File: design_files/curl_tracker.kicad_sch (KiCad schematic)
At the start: 38 parts, among them J1 JST-PH, J2 USB_C_Receptacle, J3 SSD1306 OLED, J4 JST-PH, Q1 DMP2035, Q2 AO3400A, SW1 SW_Push, SW2 SW_Push, SW3 SW_Push, U1 AP2112K-3.3, U2 ESP32-C3-MINI-1, U3 MCP73831-2-OT, U4 BMI270, U5 USBLC6-2SC6

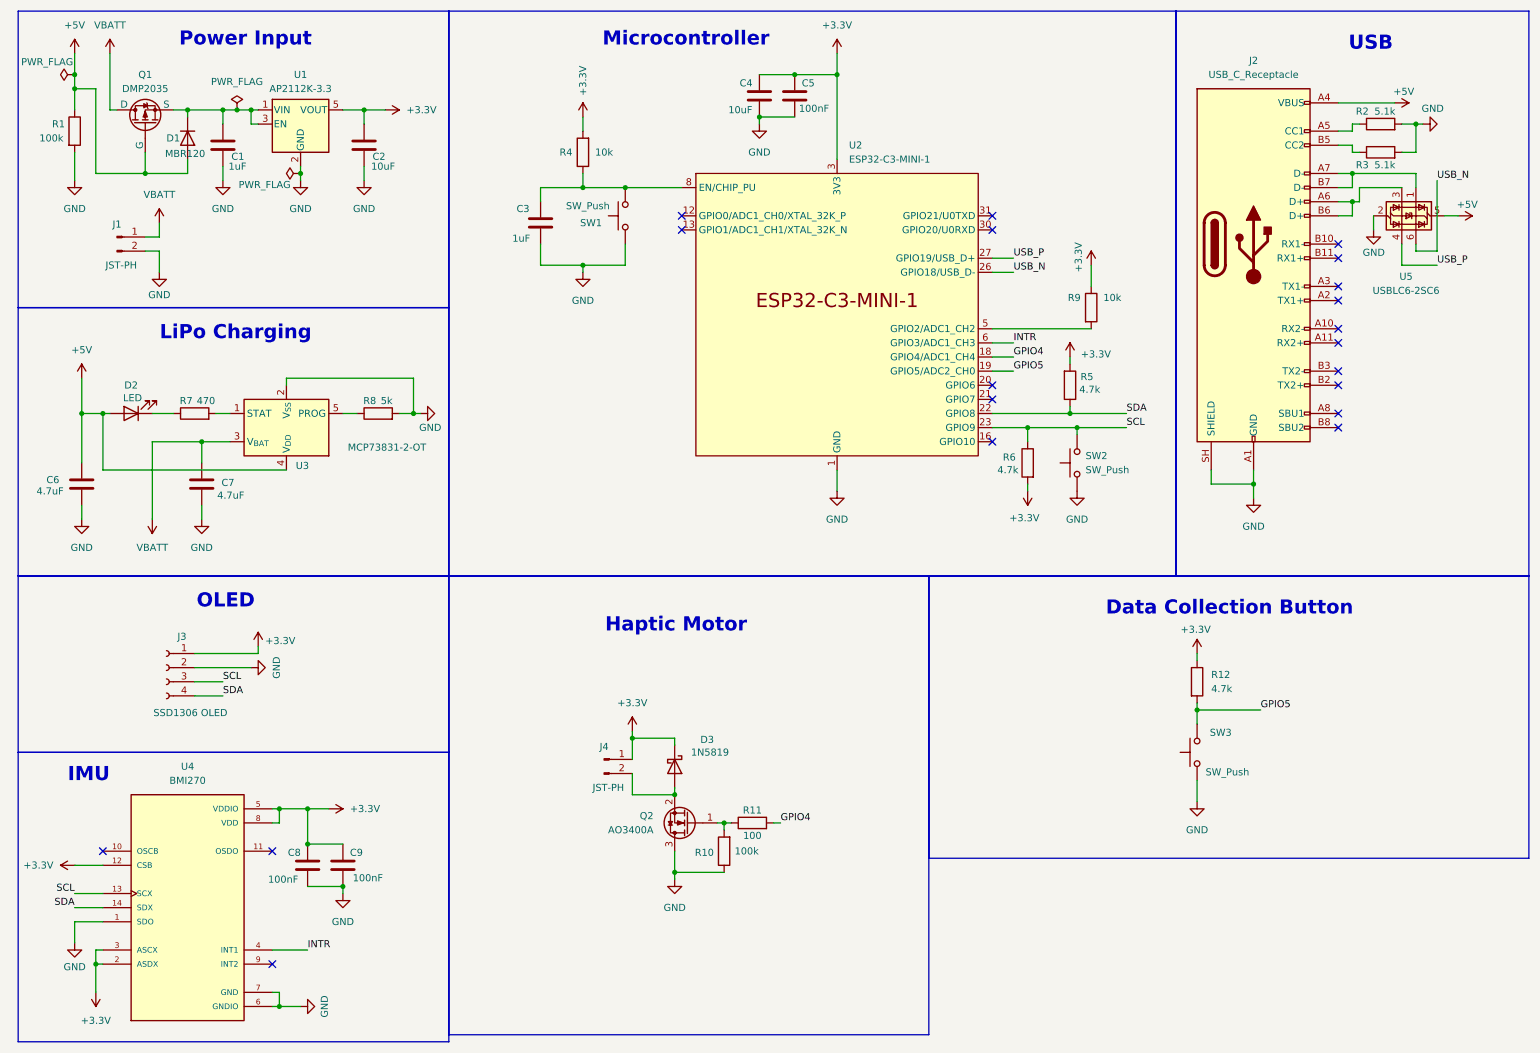
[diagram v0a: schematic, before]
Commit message: finished schematic
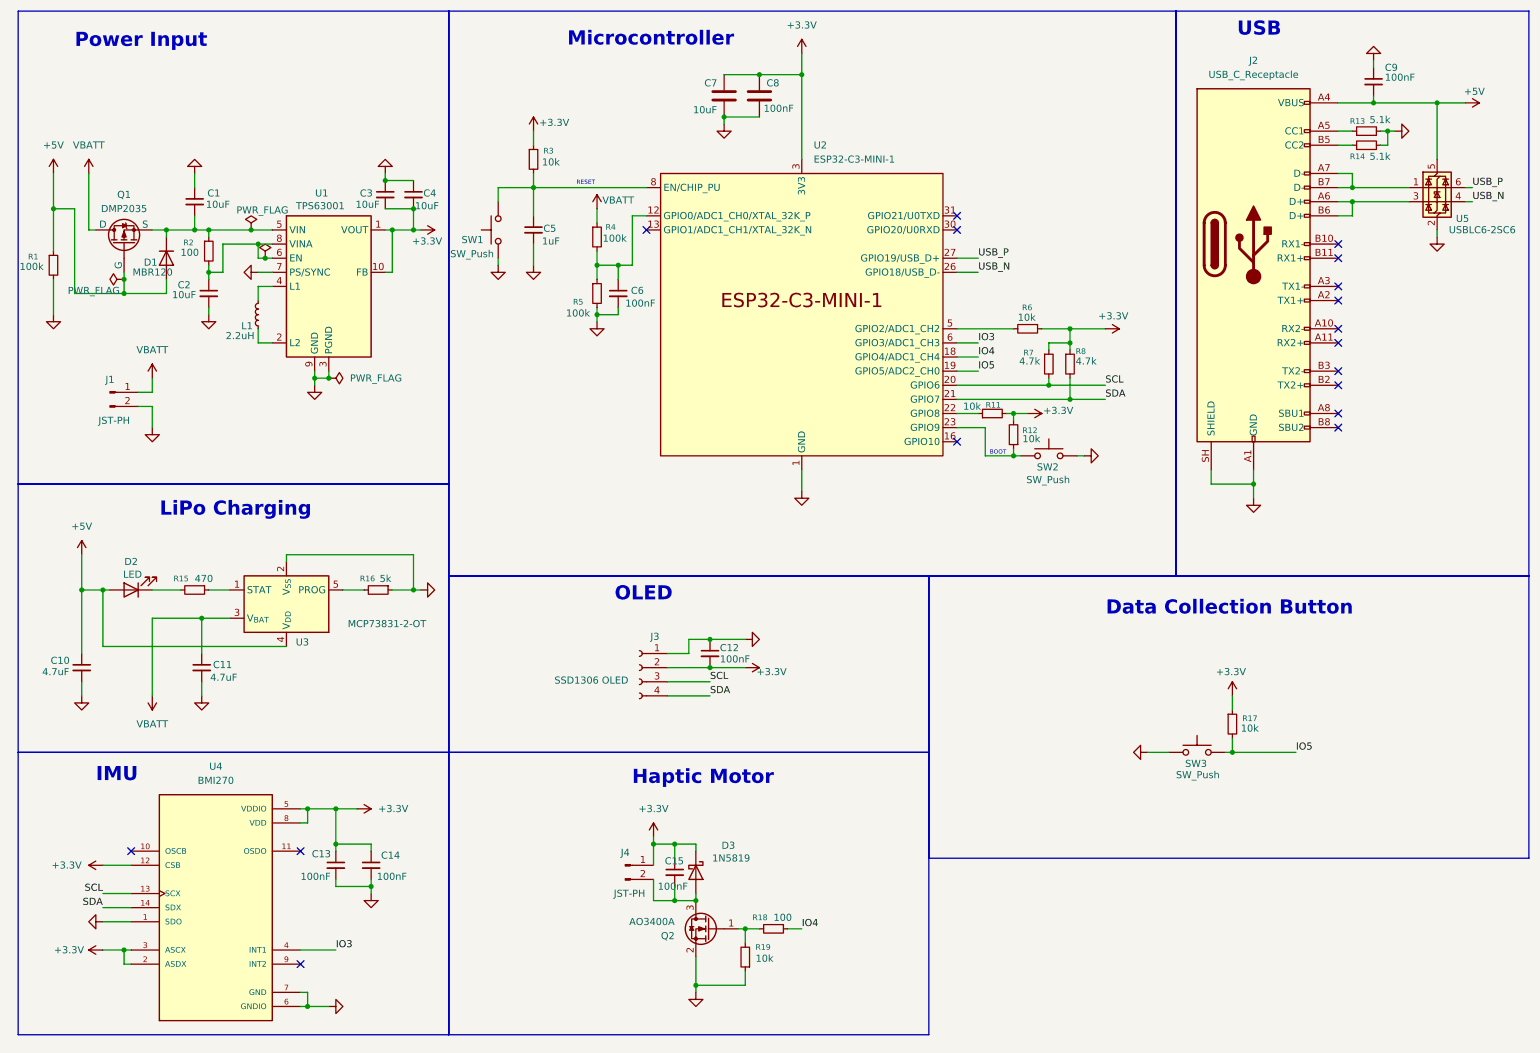
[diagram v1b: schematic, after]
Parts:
- removed C1, C3: 1uF, Capacitor_SMD:C_0402_1005Metric, symbol Device:C
- removed C2: 10uF, Capacitor_SMD:C_0805_2012Metric, symbol Device:C
- removed C6, C7: 4.7uF, Capacitor_SMD:C_0603_1608Metric, symbol Device:C
- removed C8, C9: 100nF, Capacitor_SMD:C_0402_1005Metric, symbol Device:C
- removed R1, R10: 100k, Resistor_SMD:R_0402_1005Metric, symbol Device:R
- removed R11: 100, Resistor_SMD:R_0402_1005Metric, symbol Device:R
- removed R12, R5, R6: 4.7k, Resistor_SMD:R_0402_1005Metric, symbol Device:R
- removed R2, R3: 5.1k, Resistor_SMD:R_0402_1005Metric, symbol Device:R
- removed R4, R9: 10k, Resistor_SMD:R_0402_1005Metric, symbol Device:R
- removed R7: 470, Resistor_SMD:R_0402_1005Metric, symbol Device:R
- removed R8: 5k, Resistor_SMD:R_0402_1005Metric, symbol Device:R
- removed U1: AP2112K-3.3, Package_TO_SOT_SMD:SOT-23-5, symbol Regulator_Linear:AP2112K-3.3
- removed U4: BMI270, BMI270:XDCR_BMI270, symbol BMI:BMI270
- added C1, C2, C3, C4: 10uF, Capacitor_SMD:C_0805_2012Metric, symbol Device:C_Small
- added C10, C11: 4.7uF, Capacitor_SMD:C_0805_2012Metric, symbol Device:C_Small
- added C12, C15, C6, C9: 100nF, Capacitor_SMD:C_0402_1005Metric, symbol Device:C_Small
- added C13, C14: 100nF, Capacitor_SMD:C_0805_2012Metric, symbol Device:C_Small
- added C5: 1uF, Capacitor_SMD:C_0805_2012Metric, symbol Device:C_Small
- added L1: 2.2uH, Inductor_SMD:L_Coilcraft_LPS4018, symbol Device:L_Small
- added R1, R4, R5: 100k, Resistor_SMD:R_0402_1005Metric, symbol Device:R_Small
- added R11, R12, R17, R19, R3, R6: 10k, Resistor_SMD:R_0402_1005Metric, symbol Device:R_Small
- added R13, R14: 5.1k, Resistor_SMD:R_0402_1005Metric, symbol Device:R_Small
- added R15: 470, Resistor_SMD:R_0402_1005Metric, symbol Device:R_Small
- added R16: 5k, Resistor_SMD:R_0402_1005Metric, symbol Device:R_Small
- added R18, R2: 100, Resistor_SMD:R_0402_1005Metric, symbol Device:R_Small
- added R7, R8: 4.7k, Resistor_SMD:R_0402_1005Metric, symbol Device:R_Small
- added U1: TPS63001, Package_SON:Texas_DRC0010J_ThermalVias, symbol Regulator_Switching:TPS63001
- added U4: BMI270, BMI270:XDCR_BMI270, symbol BMI270:BMI270
- D3: footprint Diode_THT:D_DO-41_SOD81_P10.16mm_Horizontal -> Diode_SMD:D_SOD-123
- SW1, SW2, SW3: footprint Button_Switch_SMD:SW_SPST_TL3342 -> Button_Switch_SMD:SW_SPST_TL3305A
- renumbered C4 to C7, C5 to C8
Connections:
- net +3.3V: now also J3.2 (Pin_2), C12.2, C13.1, C14.1, C15.1, C3.2, C4.2, R11.2, R12.2, R17.1, R3.1, R6.1, R7.1, R8.1, U1.1 (VOUT), U1.10 (FB), U4.12 (CSB), U4.2 (ASDX), U4.3 (ASCX), U4.5 (VDDIO), U4.8 (VDD); no longer J3.1 (Pin_1)
- net +5V: now also C10.1, C9.2, R1.1
- net GND: now also J3.1 (Pin_1), Q2.2 (S), SW2.2, C1.1, C10.2, C11.2, C12.1, C13.2, C14.2, C2.2, C3.1, C4.1, C5.2, C6.2, C9.1, R1.2, R13.2, R14.2, R16.1, R19.1, R5.2, U1.11 (PGND), U1.3 (PGND), U1.7 (PS/SYNC), U1.9 (GND), U4.1 (SDO), U4.6 (GNDIO), U4.7 (GND); no longer J3.2 (Pin_2), Q2.3 (D), SW2.1
- net SCL: now also U2.20 (GPIO6), R7.2, U4.13 (SCX); no longer SW2.2, U2.23 (GPIO9)
- net SDA: now also U2.21 (GPIO7), R8.2, U4.14 (SDX); no longer U2.22 (GPIO8)
- net USB_N: now also U5.4 (I/O2); no longer U5.6 (I/O1)
- net USB_P: now also U5.6 (I/O1); no longer U5.4 (I/O2)
- net VBATT: now also C11.1, R4.1
- net at D1.1 (K), Q1.3 (S): now also C1.2, R2.1, U1.5 (VIN)
- net at U2.5 (GPIO2/ADC1_CH2): now also R6.2
- net at Q2.1 (G): now also R18.2, R19.2
- net at U2.12 (GPIO0/ADC1_CH0/XTAL_32K_P): now also C6.1, R4.2, R5.1
- net at SW1.2, U2.8 (EN/CHIP_PU): now also C5.1, R3.2
- net at U3.1 (STAT): now also R15.1
- net at U3.5 (PROG): now also R16.2
- net at D3.2 (A), J4.2 (Pin_2): now also Q2.3 (D), C15.2; no longer Q2.2 (S)
- net at J2.A5 (CC1): now also R13.1
- net at J2.B5 (CC2): now also R14.1
- net at D2.1 (K): now also R15.2
- net GPIO4 renamed IO4
- net IO4: now also R18.1
- net GPIO5 renamed IO5
- net IO5: now also R17.2
- net INTR renamed IO3
- net IO3: now also U4.4 (INT1)
- new net: L1.1, U1.2 (L2)
- new net: L1.2, U1.4 (L1)
- new net: R11.1, U2.22 (GPIO8)
- new net: R12.1, SW2.1, U2.23 (GPIO9)
- new net: C2.1, R2.2, U1.6 (EN), U1.8 (VINA)
- no-connect marks 20 -> 17
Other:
- note added: "BOOT"
- note added: "RESET"
- moved on the sheet: C7, C8, D1, D2, D3, J1, J3, J4, Q1, Q2, SW1, SW2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

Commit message: finished schematic
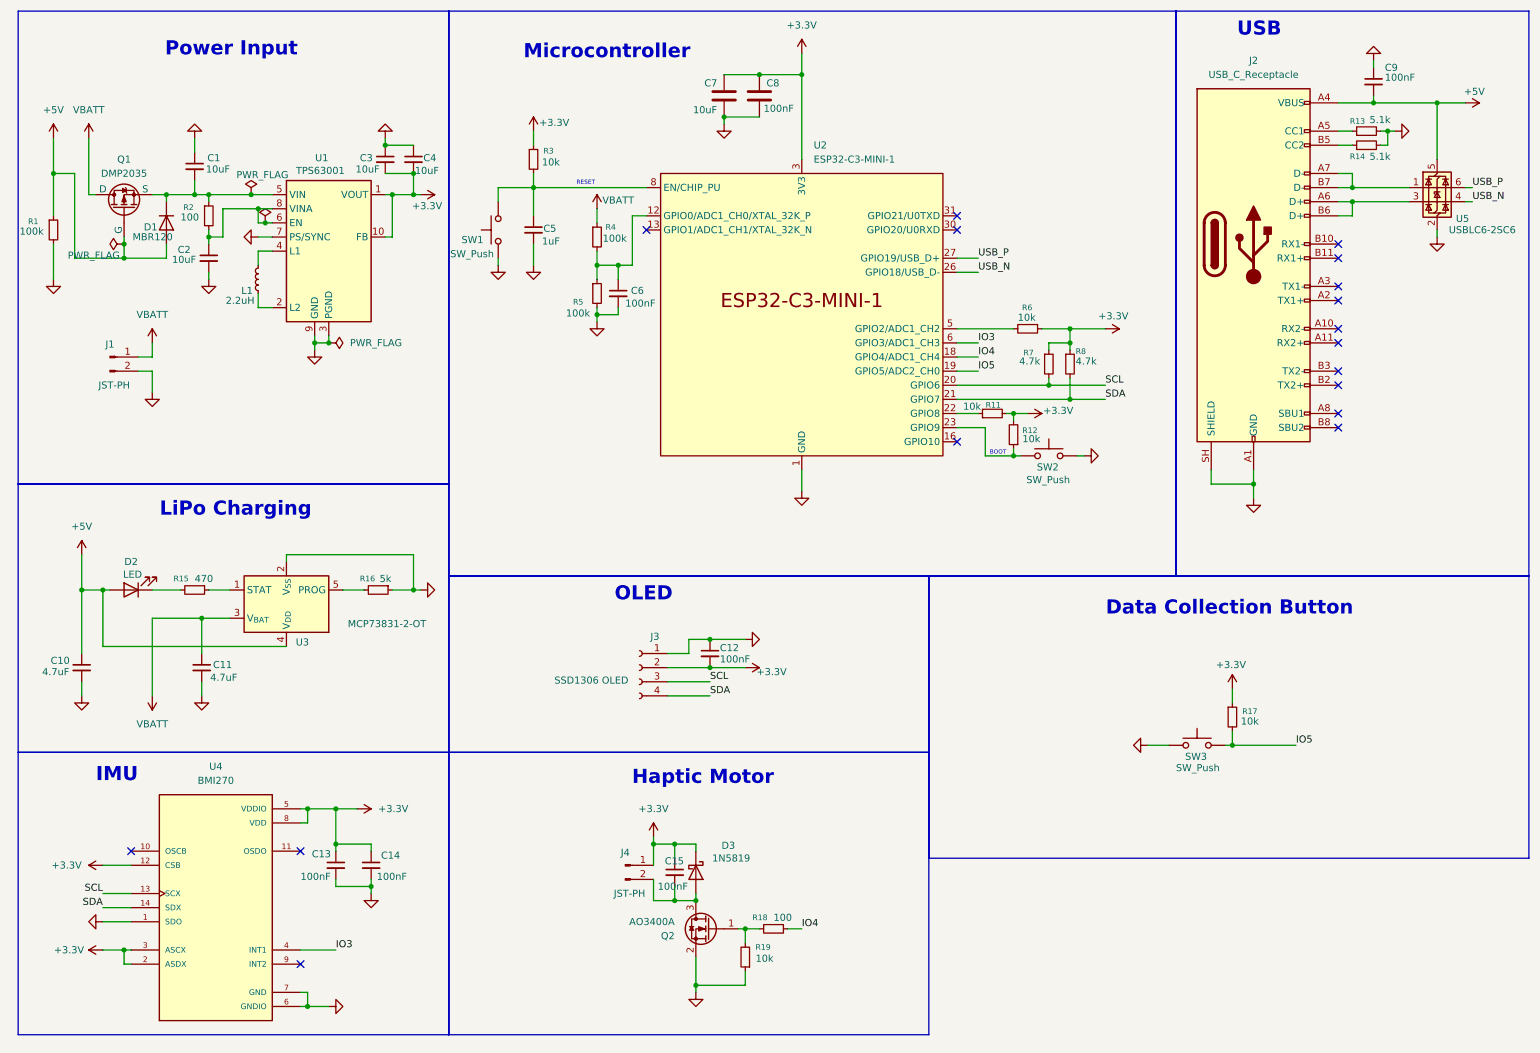
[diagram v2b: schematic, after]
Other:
- moved on the sheet: C1, C2, C3, C4, D1, J1, L1, Q1, R1, R17, R2, SW3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
